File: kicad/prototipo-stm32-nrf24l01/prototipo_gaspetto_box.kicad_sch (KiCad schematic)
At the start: 19 parts, among them U1 YAAJ_BluePill_Part_Like_SWD_B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, U10 DRV5033AJxLPG, U11 DRV5033AJxLPG, U12 DRV5033AJxLPG, U13 DRV5033AJxLPG, U14 DRV5033AJxLPG, U15 DRV5033AJxLPG, U16 DRV5033AJxLPG, U17 DRV5033AJxLPG, U18 DRV5033AJxLPG, U19 DRV5033AJxLPG, U2 nRF24L01+, U3 PCF8575DBR, U4 DRV5033AJxLPG, U5 DRV5033AJxLPG, U6 DRV5033AJxLPG, U7 DRV5033AJxLPG, U8 DRV5033AJxLPG, U9 DRV5033AJxLPG

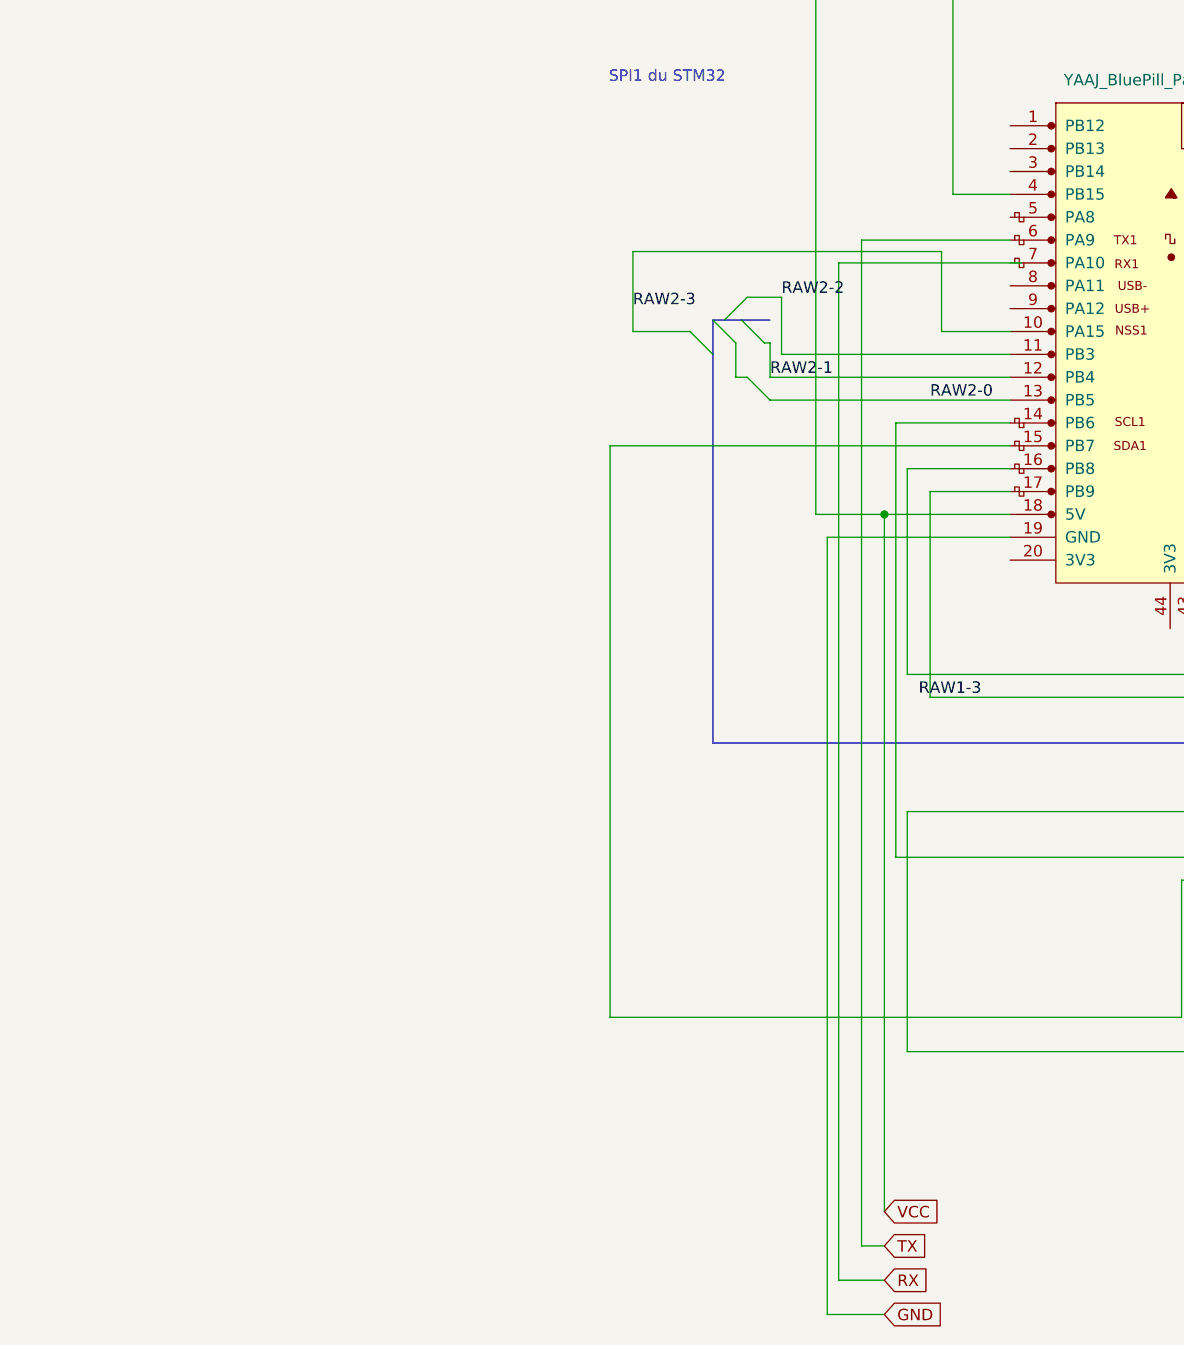
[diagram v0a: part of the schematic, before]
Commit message: kicad: clean projects
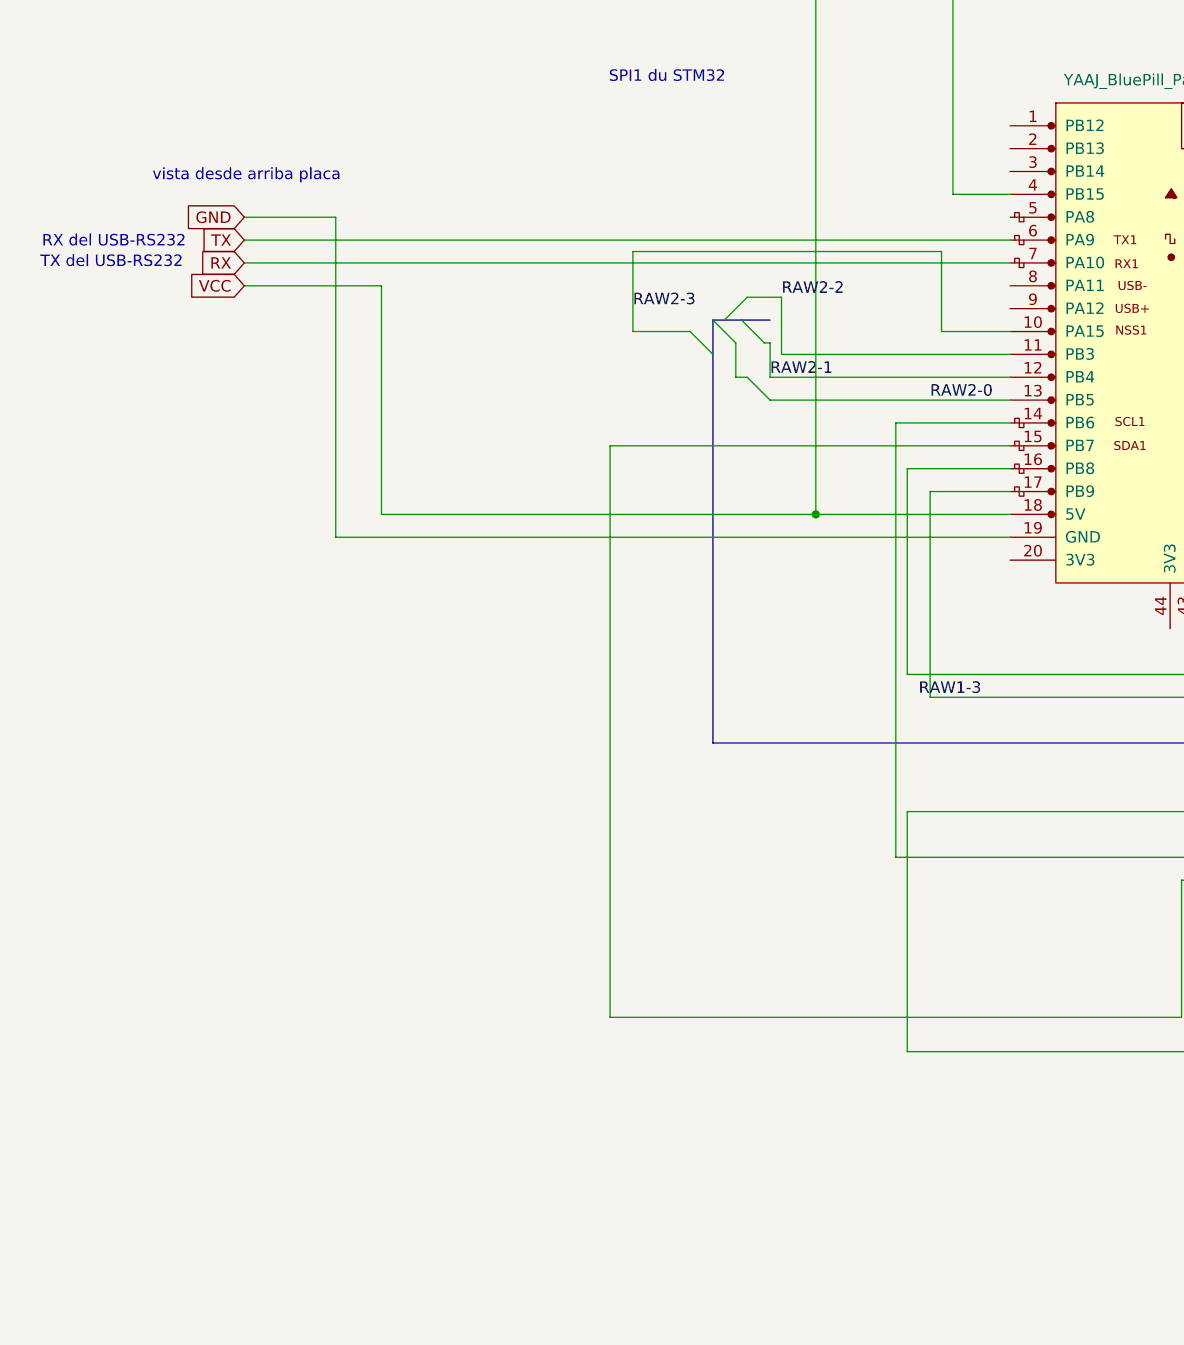
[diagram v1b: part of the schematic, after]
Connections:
- net RX: now also U1.7 (PA10)
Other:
- note added: "RX del USB-RS232"
- note added: "TX del USB-RS232"
- note added: "vista desde arriba placa"
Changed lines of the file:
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@@
 	)
 	(junction
-		(at 138.43 144.78)
+		(at 130.81 144.78)
 		(diameter 0)
 		(color 0 0 0 0)
@@
 	(wire
 		(pts
-			(xy 132.08 147.32) (xy 132.08 233.68)
-		)
-		(stroke
-			(width 0)
-			(type default)
-		)
-	)
-	(wire
-		(pts
 			(xy 107.95 200.66) (xy 171.45 200.66)
 		)
@@
 	(wire
 		(pts
+			(xy 82.55 144.78) (xy 130.81 144.78)
+		)
+		(stroke
+			(width 0)
+			(type default)
+		)
+	)
+	(wire
+		(pts
 			(xy 203.2 114.3) (xy 198.12 114.3)
 		)
@@
 	(wire
 		(pts
-			(xy 322.58 133.35) (xy 322.58 114.3)
+			(xy 67.31 111.76) (xy 77.47 111.76)
 		)
 		(stroke
@@
 	(wire
 		(pts
-			(xy 378.46 179.07) (xy 378.46 185.42)
+			(xy 322.58 133.35) (xy 322.58 114.3)
 		)
 		(stroke
@@
 	(wire
 		(pts
-			(xy 152.4 144.78) (xy 138.43 144.78)
+			(xy 378.46 179.07) (xy 378.46 185.42)
 		)
 		(stroke
@@
 	(wire
 		(pts
-			(xy 133.35 116.84) (xy 153.67 116.84)
+			(xy 328.93 179.07) (xy 328.93 184.15)
 		)
 		(stroke
@@
 	(wire
 		(pts
-			(xy 328.93 179.07) (xy 328.93 184.15)
+			(xy 394.97 67.31) (xy 394.97 82.55)
 		)
 		(stroke
@@
 	(wire
 		(pts
-			(xy 394.97 67.31) (xy 394.97 82.55)
+			(xy 316.23 184.15) (xy 316.23 124.46)
 		)
 		(stroke
@@
 	(wire
 		(pts
-			(xy 316.23 184.15) (xy 316.23 124.46)
+			(xy 394.97 104.14) (xy 394.97 114.3)
 		)
 		(stroke
@@
 	(wire
 		(pts
-			(xy 394.97 104.14) (xy 394.97 114.3)
+			(xy 369.57 124.46) (xy 369.57 95.25)
 		)
 		(stroke
@@
 	(wire
 		(pts
-			(xy 369.57 124.46) (xy 369.57 95.25)
+			(xy 82.55 144.78) (xy 82.55 119.38)
 		)
 		(stroke
@@
 	(wire
 		(pts
-			(xy 394.97 168.91) (xy 394.97 152.4)
+			(xy 77.47 111.76) (xy 77.47 147.32)
 		)
 		(stroke
@@
 	(wire
 		(pts
-			(xy 132.08 233.68) (xy 138.43 233.68)
+			(xy 394.97 168.91) (xy 394.97 152.4)
 		)
 		(stroke
@@
 	(wire
 		(pts
-			(xy 152.4 114.3) (xy 135.89 114.3)
-		)
-		(stroke
-			(width 0)
-			(type default)
-		)
-	)
-	(wire
-		(pts
 			(xy 394.97 82.55) (xy 394.97 104.14)
 		)
@@
 	(wire
 		(pts
-			(xy 133.35 229.87) (xy 133.35 116.84)
-		)
-		(stroke
-			(width 0)
-			(type default)
-		)
-	)
-	(wire
-		(pts
-			(xy 138.43 229.87) (xy 133.35 229.87)
-		)
-		(stroke
-			(width 0)
-			(type default)
-		)
-	)
-	(wire
-		(pts
 			(xy 201.93 204.47) (xy 140.97 204.47)
 		)
@@
 	(wire
 		(pts
+			(xy 82.55 119.38) (xy 67.31 119.38)
+		)
+		(stroke
+			(width 0)
+			(type default)
+		)
+	)
+	(wire
+		(pts
 			(xy 121.92 129.54) (xy 123.19 129.54)
 		)
@@
 	(wire
 		(pts
-			(xy 138.43 144.78) (xy 138.43 222.25)
-		)
-		(stroke
-			(width 0)
-			(type default)
-		)
-	)
-	(wire
-		(pts
 			(xy 125.095 125.73) (xy 125.73 125.73)
 		)
@@
 	(wire
 		(pts
-			(xy 138.43 144.78) (xy 130.81 144.78)
+			(xy 130.81 144.78) (xy 152.4 144.78)
 		)
 		(stroke
@@
 	(wire
 		(pts
+			(xy 67.31 116.84) (xy 152.4 116.84)
+		)
+		(stroke
+			(width 0)
+			(type default)
+		)
+	)
+	(wire
+		(pts
 			(xy 280.67 118.11) (xy 280.67 132.08)
 		)
@@
 		)
 	)
-	(bus
+	(wire
 		(pts
-			(xy 280.67 111.76) (xy 288.29 111.76)
+			(xy 67.31 114.3) (xy 152.4 114.3)
 		)
 		(stroke
@@
 		)
 	)
-	(wire
+	(bus
 		(pts
-			(xy 344.17 185.42) (xy 340.36 185.42)
+			(xy 280.67 111.76) (xy 288.29 111.76)
 		)
 		(stroke
@@
 	(wire
 		(pts
-			(xy 283.21 188.595) (xy 283.21 190.5)
+			(xy 344.17 185.42) (xy 340.36 185.42)
 		)
 		(stroke
@@
 	(wire
 		(pts
-			(xy 200.66 95.25) (xy 200.66 111.76)
+			(xy 283.21 188.595) (xy 283.21 190.5)
 		)
 		(stroke
@@
 	(wire
 		(pts
-			(xy 273.685 114.3) (xy 283.21 114.3)
+			(xy 200.66 95.25) (xy 200.66 111.76)
 		)
 		(stroke
@@
 	(wire
 		(pts
-			(xy 135.89 114.3) (xy 135.89 226.06)
+			(xy 273.685 114.3) (xy 283.21 114.3)
 		)
 		(stroke
@@
 		)
 	)
-	(wire
-		(pts
-			(xy 135.89 226.06) (xy 138.43 226.06)
-		)
-		(stroke
-			(width 0)
-			(type default)
-		)
-	)
 	(bus
 		(pts
@@
 	(wire
 		(pts
-			(xy 152.4 147.32) (xy 132.08 147.32)
+			(xy 152.4 147.32) (xy 77.47 147.32)
 		)
 		(stroke
@@
 		)
 	)
+	(text "vista desde arriba placa"
+		(exclude_from_sim no)
+		(at 67.564 107.188 0)
+		(effects
+			(font
+				(size 1.27 1.27)
+			)
+		)
+	)
+	(text "RX del USB-RS232"
+		(exclude_from_sim no)
+		(at 52.832 114.554 0)
+		(effects
+			(font
+				(size 1.27 1.27)
+			)
+		)
+	)
+	(text "TX del USB-RS232"
+		(exclude_from_sim no)
+		(at 52.578 116.84 0)
+		(effects
+			(font
+				(size 1.27 1.27)
+			)
+		)
+	)
 	(text "SPI1 du STM32"
 		(exclude_from_sim no)
@@
 	(global_label "TX"
 		(shape input)
-		(at 138.43 226.06 0)
+		(at 67.31 114.3 180)
 		(fields_autoplaced yes)
 		(effects
@@
 				(size 1.27 1.27)
 			)
-			(justify left)
+			(justify right)
 		)
 		(property "Intersheetrefs" "${INTERSHEET_REFS}"
-			(at 143.5923 226.06 0)
+			(at 62.1477 114.3 0)
 			(effects
 				(font
 					(size 1.27 1.27)
 				)
-				(justify left)
+				(justify right)
 				(hide yes)
 			)
@@
 	(global_label "VCC"
 		(shape input)
-		(at 138.43 222.25 0)
+		(at 67.31 119.38 180)
 		(fields_autoplaced yes)
 		(effects
@@
 				(size 1.27 1.27)
 			)
-			(justify left)
+			(justify right)
 		)
 		(property "Intersheetrefs" "${INTERSHEET_REFS}"
-			(at 145.0438 222.25 0)
+			(at 60.6962 119.38 0)
 			(effects
 				(font
 					(size 1.27 1.27)
 				)
-				(justify left)
+				(justify right)
 				(hide yes)
 			)
@@
 	(global_label "RX"
 		(shape input)
-		(at 138.43 229.87 0)
+		(at 67.31 116.84 180)
 		(fields_autoplaced yes)
 		(effects
@@
 				(size 1.27 1.27)
 			)
-			(justify left)
+			(justify right)
 		)
 		(property "Intersheetrefs" "${INTERSHEET_REFS}"
-			(at 143.8947 229.87 0)
+			(at 61.8453 116.84 0)
 			(effects
 				(font
 					(size 1.27 1.27)
 				)
-				(justify left)
+				(justify right)
 				(hide yes)
 			)
@@
 	(global_label "GND"
 		(shape input)
-		(at 138.43 233.68 0)
+		(at 67.31 111.76 180)
 		(fields_autoplaced yes)
 		(effects
@@
 				(size 1.27 1.27)
 			)
-			(justify left)
+			(justify right)
 		)
 		(property "Intersheetrefs" "${INTERSHEET_REFS}"
-			(at 145.2857 233.68 0)
+			(at 60.4543 111.76 0)
 			(effects
 				(font
 					(size 1.27 1.27)
 				)
-				(justify left)
+				(justify right)
 				(hide yes)
 			)

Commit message: feat: add gaspetto box sch
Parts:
- removed U1: YAAJ_BluePill_Part_Like_SWD_Breakout, symbol YAAJ_BluePill_Part_Like_SWD_Breakout:YAAJ_BluePill_Part_Like_SWD_Breakout
- removed U10, U15, U4, U5: DRV5033AJxLPG, Package_TO_SOT_THT:TO-92_Inline, symbol Sensor_Magnetic:DRV5033AJxLPG
- removed U3: PCF8575DBR, Package_SO:SSOP-24_5.3x8.2mm_P0.65mm, symbol Interface_Expansion:PCF8575DBR
- added C1: 100nF, Capacitor_THT:CP_Axial_L10.0mm_D4.5mm_P15.00mm_Horizontal, symbol Device:C
- added C10, C12, C5, C6: 100nF, Capacitor_THT:CP_Radial_D4.0mm_P1.50mm, symbol Device:C
- added C11, C9: 10uF, Capacitor_THT:C_Radial_D8.0mm_H11.5mm_P3.50mm, symbol Device:C_Polarized
- added C2, C4, C8: 1uF, Capacitor_THT:C_Radial_D8.0mm_H11.5mm_P3.50mm, symbol Device:C
- added C7: 470Uf, Capacitor_THT:C_Radial_D8.0mm_H11.5mm_P3.50mm, symbol Device:C_Polarized
- added D1, D2, D3: APA-106-F5, LED_THT:LED_D5.0mm-4_RGB, symbol LED:APA-106-F5
- added J1: UPS IN, Connector_PinHeader_1.27mm:PinHeader_1x02_P1.27mm_Horizontal, symbol Connector_Generic:Conn_01x02
- added J2, J5, J6: Conn_02x05_Odd_Even, Connector_PinHeader_1.27mm:PinHeader_2x05_P1.27mm_Vertical, symbol Connector_Generic:Conn_02x05_Odd_Even
- added J3: UPS OUT, Connector_PinHeader_1.27mm:PinHeader_1x02_P1.27mm_Vertical, symbol Connector_Generic:Conn_01x02
- added J4, J7: Conn_01x11, Connector_PinHeader_1.27mm:PinHeader_1x11_P1.27mm_Vertical, symbol Connector_Generic:Conn_01x11
- added P1: USB_C_Plug_USB2.0, Connector_USB:USB_C_Receptacle_XKB_U262-16XN-4BVC11, symbol Connector:USB_C_Plug_USB2.0
- added Q1, Q2: AO3401A, Package_TO_SOT_SMD:SOT-23, symbol Transistor_FET:AO3401A
- added R1, R5: 10k, Resistor_THT:R_Axial_DIN0309_L9.0mm_D3.2mm_P12.70mm_Horizontal, symbol Device:R
- added R2, R4: 100k, Resistor_THT:R_Axial_DIN0309_L9.0mm_D3.2mm_P12.70mm_Horizontal, symbol Device:R
- added R3: 5k1, Resistor_THT:R_Axial_DIN0309_L9.0mm_D3.2mm_P12.70mm_Horizontal, symbol Device:R
- added R6: 330, Resistor_THT:R_Axial_DIN0309_L9.0mm_D3.2mm_P12.70mm_Horizontal, symbol Device:R
- added U10, U15, U20, U25, U4: ADS1115IDGS, Package_SO:TSSOP-10_3x3mm_P0.5mm, symbol Analog_ADC:ADS1115IDGS
- added U21, U22, U23, U24, U26, U27, U28, U29: DRV5033AJxLPG, Package_TO_SOT_THT:TO-92_Inline, symbol Sensor_Magnetic:DRV5033AJxLPG
- added U3, U30, U5: MCP1700x-330xxTO, Package_TO_SOT_THT:TO-92_Inline, symbol Regulator_Linear:MCP1700x-330xxTO
- added U31: YAAJ_WeAct_BlackPill_Part_Like_SWD_Breakout, Package_DIP:DIP-40_W25.4mm_LongPads, symbol YAAJ_WeAct_BlackPill_Part_Like_SWD_Breakout:YAAJ_WeAct_BlackPill_Part_Like_SWD_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
- U2: footprint MODULE -> Connector_PinHeader_2.54mm:PinHeader_2x04_P2.54mm_Vertical
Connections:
- net RAW0-0 is gone; now on net GND: U6.2 (GND), U7.2 (GND)
- net RAW1-0 is gone; now on net GND: U11.2 (GND)
- net RAW1-2 is gone; now on net GND: U9.2 (GND)
- net RAW1-3 is gone; now on net GND: U8.2 (GND)
- net RAW2-0 is gone; now on net GND: U19.2 (GND)
- net RAW2-2 is gone; now on net GND: U17.2 (GND)
- net RAW2-3 is gone; now on net GND: U16.2 (GND)
- net GND: now also U12.2 (GND), U13.2 (GND), U14.2 (GND), U18.2 (GND), U2.1 (GND), C1.2, C10.2, C11.2, C12.2, C2.2, C4.2, C5.2, C6.2, C7.2, C8.2, C9.2, D1.2 (GND), D2.2 (GND), D3.2 (GND), J1.1 (Pin_1), J2.3 (Pin_3), J2.6 (Pin_6), J3.1 (Pin_1), J4.10 (Pin_10), J4.2 (Pin_2), J4.4 (Pin_4), J4.6 (Pin_6), J4.8 (Pin_8), J5.3 (Pin_3), J5.6 (Pin_6), J7.10 (Pin_10), J7.2 (Pin_2), J7.4 (Pin_4), J7.6 (Pin_6), J7.8 (Pin_8), P1.A1 (GND), P1.A12 (GND), P1.B1 (GND), P1.B12 (GND), R3.2, U10.3 (GND), U15.3 (GND), U20.1 (ADDR), U20.3 (GND), U21.2 (GND), U22.2 (GND), U23.2 (GND), U24.2 (GND), U25.3 (GND), U26.2 (GND), U27.2 (GND), U28.2 (GND), U29.2 (GND), U3.1 (GND), U30.1 (GND), U31.39 (GND), U4.1 (ADDR), U4.3 (GND), U5.1 (GND)
- net CSN: now reaches U2.4 (CSN)
- net CSN: now also J4.3 (Pin_3), J7.1 (Pin_1), U31.30 (PA4)
- net SCK: now reaches U2.5 (SCK)
- net SCK: now also J4.7 (Pin_7), J7.7 (Pin_7), U31.31 (PA5)
- net MISO: now reaches U2.7 (MISO)
- net MISO: now also J4.5 (Pin_5), J7.5 (Pin_5), U31.32 (PA6)
- net MOSI: now reaches U2.6 (MOSI)
- net MOSI: now also J4.1 (Pin_1), J7.3 (Pin_3), U31.33 (PA7)
- net CE: now reaches U2.3 (CE)
- net CE: now also J4.9 (Pin_9), J7.9 (Pin_9), U31.29 (PA3)
- net VCC renamed 3V3_SWITCHED
- net 3V3_SWITCHED: now also J2.2 (Pin_2), J5.2 (Pin_2), Q2.3 (D), U10.8 (VDD), U15.8 (VDD), U20.8 (VDD), U21.1 (VCC), U22.1 (VCC), U23.1 (VCC), U24.1 (VCC), U25.1 (ADDR), U25.8 (VDD), U26.1 (VCC), U27.1 (VCC), U28.1 (VCC), U29.1 (VCC), U4.8 (VDD); no longer U2.2 (VCC)
- new net: D1.4 (DI), D2.1 (DO)
- new net: R1.1, U31.3 (PB14)
- new net: R5.1, U31.4 (PB15)
- new net: P1.A7 (D-), U31.8 (PA11)
- new net: P1.A6 (D+), U31.9 (PA12)
- new net: U10.7 (AIN3), U11.3 (OUT)
- new net: U24.3 (OUT), U25.4 (AIN0)
- new net: U23.3 (OUT), U25.5 (AIN1)
- new net: U22.3 (OUT), U25.6 (AIN2)
- new net: U21.3 (OUT), U25.7 (AIN3)
- new net: C10.1, Q2.1 (G), R2.1, R5.2
- new net: U10.4 (AIN0), U14.3 (OUT)
- new net: U4.5 (AIN1), U8.3 (OUT)
- new net: U10.5 (AIN1), U13.3 (OUT)
- new net: U10.6 (AIN2), U12.3 (OUT)
- new net: U15.5 (AIN1), U18.3 (OUT)
- new net: C1.1, Q1.1 (G), R1.2, R4.1
- new net: U15.6 (AIN2), U17.3 (OUT)
- new net: U4.7 (AIN3), U6.3 (OUT)
- new net: U20.4 (AIN0), U29.3 (OUT)
- new net: U20.5 (AIN1), U28.3 (OUT)
- new net: U20.6 (AIN2), U27.3 (OUT)
- new net: U20.7 (AIN3), U26.3 (OUT)
- new net: P1.A5 (CC), R3.1
- new net: J1.2 (Pin_2), P1.A4 (VBUS), P1.A9 (VBUS), P1.B4 (VBUS), P1.B9 (VBUS)
- new net: U4.4 (AIN0), U9.3 (OUT)
- new net: U4.6 (AIN2), U7.3 (OUT)
- new net: U15.7 (AIN3), U16.3 (OUT)
- new net: U15.4 (AIN0), U19.3 (OUT)
- new net: D2.4 (DI), D3.1 (DO)
- new net: D3.4 (DI), R6.2
- new net 3V3_PRE_SWITCHED: C7.1, Q2.2 (S), R2.2, U3.3 (VO)
- new net 3v3_ALWAYS: C9.1, U31.38 (3V3), U5.3 (VO)
- new net 3v3_NRF: C11.1, C2.1, U2.2 (VCC), U30.3 (VO)
- new net 5V_ALWAYS: C4.1, C8.1, J3.2 (Pin_2), J4.11 (Pin_11), J7.11 (Pin_11), Q1.2 (S), R4.2, U3.2 (VI), U30.2 (VI), U5.2 (VI)
- new net 5V_SWITCHED: C12.1, C5.1, C6.1, D1.3 (VDD), D2.3 (VDD), D3.3 (VDD), J2.1 (Pin_1), J5.1 (Pin_1), Q1.3 (D)
- new net I2C1_SCL: J2.5 (Pin_5), J5.5 (Pin_5), U10.10 (SCL), U15.1 (ADDR), U15.10 (SCL), U25.10 (SCL), U31.14 (PB6), U4.10 (SCL)
- new net I2C1_SDA: J2.4 (Pin_4), J5.4 (Pin_4), U10.1 (ADDR), U10.9 (SDA), U15.9 (SDA), U25.9 (SDA), U31.15 (PB7), U4.9 (SDA)
- new net I2C3_SCL: J2.8 (Pin_8), J5.8 (Pin_8), U20.10 (SCL), U31.5 (PA8)
- new net I2C3_SDA: J2.7 (Pin_7), J5.7 (Pin_7), U20.9 (SDA), U31.12 (PB4)
- new net LED_DATA: J2.10 (Pin_10), J5.10 (Pin_10), R6.1, U31.16 (PB8)
- new net WAKE_BUTTON: J2.9 (Pin_9), J5.9 (Pin_9), U31.17 (PB9)
- no-connect marks 0 -> 38
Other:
- note added: "A"
- note added: "ADS1115 breakboard"
- note added: "Addr=GND"
- note added: "Addr=SCL"
- note added: "Addr=SDA"
- note added: "Addr=VCC"
- note added: "B"
- note added: "C"
- note added: "Cache"
- note added: "D"
- note added: "E"
- note added: "I2C1"
- note added: "I2C3"
- note added: "PB14"
- note added: "PB15"
- note added: "Plaque NRF"
- note added: "Plaque Uc"
- note added: "To NRF module"
- note added: "Top view"
- note removed: "RX del USB-RS232"
- note removed: "SPI1 du STM32"
- note removed: "TX del USB-RS232"
- note removed: "vista desde arriba placa"
- moved on the sheet: U2
